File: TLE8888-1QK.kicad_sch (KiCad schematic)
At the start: 8 parts, among them Q1 IPD30N06S2L-23

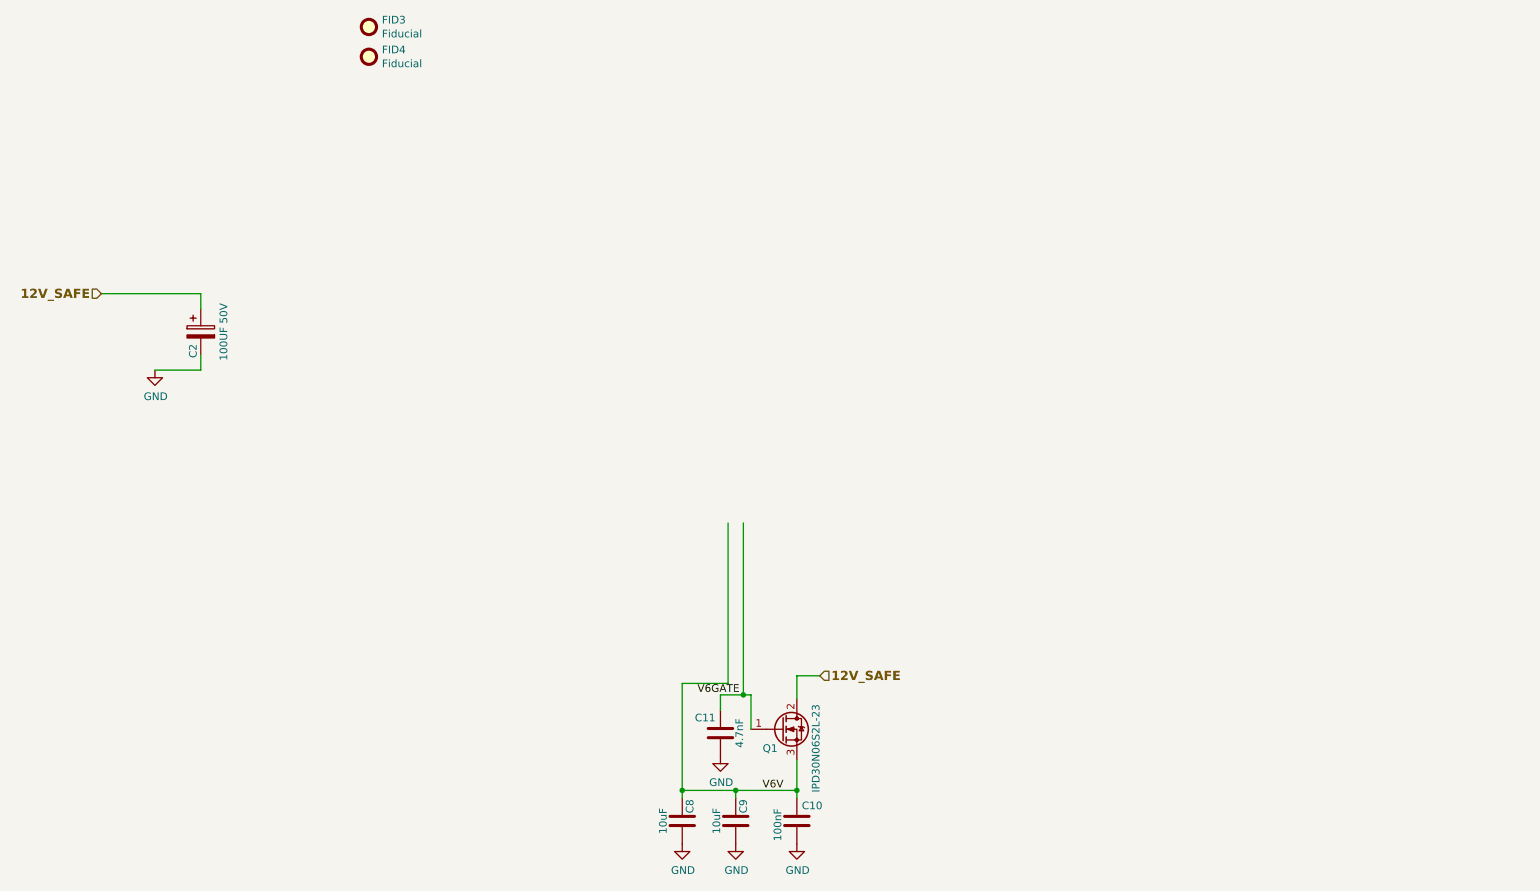
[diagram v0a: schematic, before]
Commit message: First commit
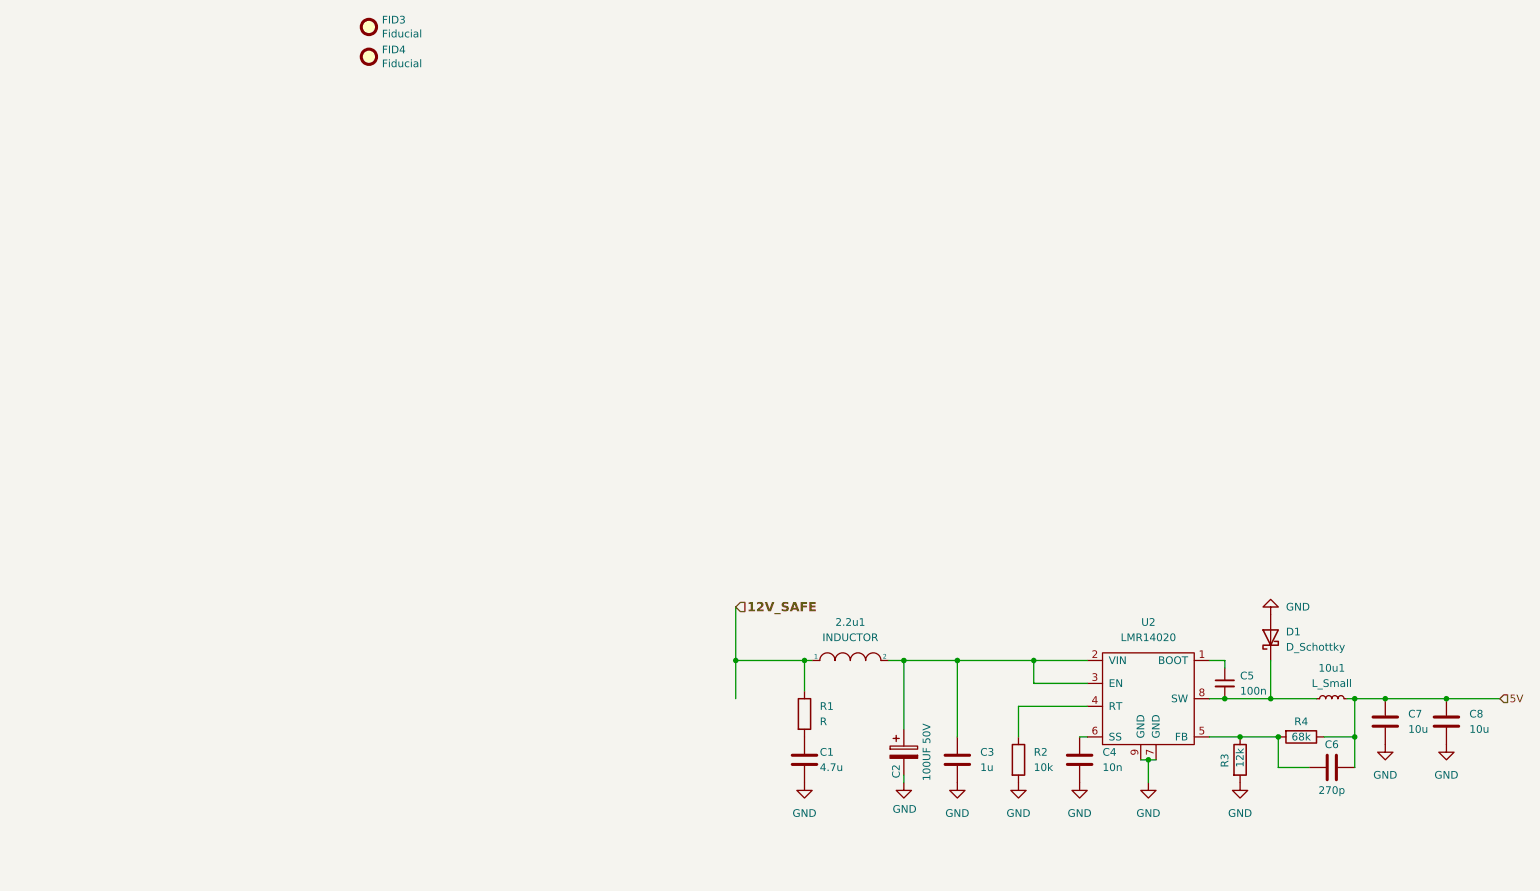
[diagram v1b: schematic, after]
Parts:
- removed C10: 100nF, Capacitor_SMD:C_0603_1608Metric, symbol Device:C
- removed C11: 4.7nF, Capacitor_SMD:C_0603_1608Metric, symbol Device:C
- removed C9: 10uF, Capacitor_SMD:C_0603_1608Metric, symbol Device:C
- removed Q1: IPD30N06S2L-23, Package_TO_SOT_SMD:TO-252-2, symbol Transistor_FET:BUZ11
- added 10u1: L_Small, symbol Device:L_Small
- added 2.2u1: INDUCTOR, symbol pspice:INDUCTOR
- added C1: 4.7u, Capacitor_SMD:C_0603_1608Metric, symbol Device:C
- added C3: 1u, Capacitor_SMD:C_0603_1608Metric, symbol Device:C
- added C4: 10n, Capacitor_SMD:C_0603_1608Metric, symbol Device:C
- added C5: 100n, symbol Device:C_Small
- added C6: 270p, Capacitor_SMD:C_0603_1608Metric, symbol Device:C
- added C7: 10u, Capacitor_SMD:C_0603_1608Metric, symbol Device:C
- added D1: D_Schottky, symbol Device:D_Schottky
- added R1: R, symbol Device:R
- added R2: 10k, Resistor_SMD:R_0402_1005Metric, symbol Device:R
- added R3: 12k, Resistor_SMD:R_0402_1005Metric, symbol Device:R
- added R4: 68k, Resistor_SMD:R_0402_1005Metric, symbol Device:R
- added U2: LMR14020, Simon:SOIC8-DFN, symbol Simon:LMR14020
- C8: value 10uF -> 10u; LCSC C19702 -> (none); Manufacturer TDK -> (none); Part # C1608X5R1E106M080AC -> (none); VEND DIGI -> (none); VEND# 445-9015-1-ND -> (none)
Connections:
- net 12V_SAFE: now also 2.2u1.1, R1.1; no longer C2.1
- net GND: now also C1.2, C3.2, C4.2, C7.2, D1.2 (A), R2.2, R3.2, U2.7 (GND), U2.9 (GND)
- net V6V renamed 5V
- net 5V: now also 10u1.2, C6.1, C7.1, R4.1
- new net: 2.2u1.2, C2.1, C3.1, U2.2 (VIN), U2.3 (EN)
- new net: C5.1, U2.1 (BOOT)
- new net: 10u1.1, C5.2, D1.1 (K), U2.8 (SW)
- new net: C1.1, R1.2
- new net: C6.2, R3.1, R4.2, U2.5 (FB)
- new net: R2.1, U2.4 (RT)
- new net: C4.1, U2.6 (SS)
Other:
- moved on the sheet: C2
